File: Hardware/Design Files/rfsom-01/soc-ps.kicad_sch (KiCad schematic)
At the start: 50 parts, among them J9 DM3CS-SF, U5 XC7Z010-1CLG400C, U7 TXS02612RTWR

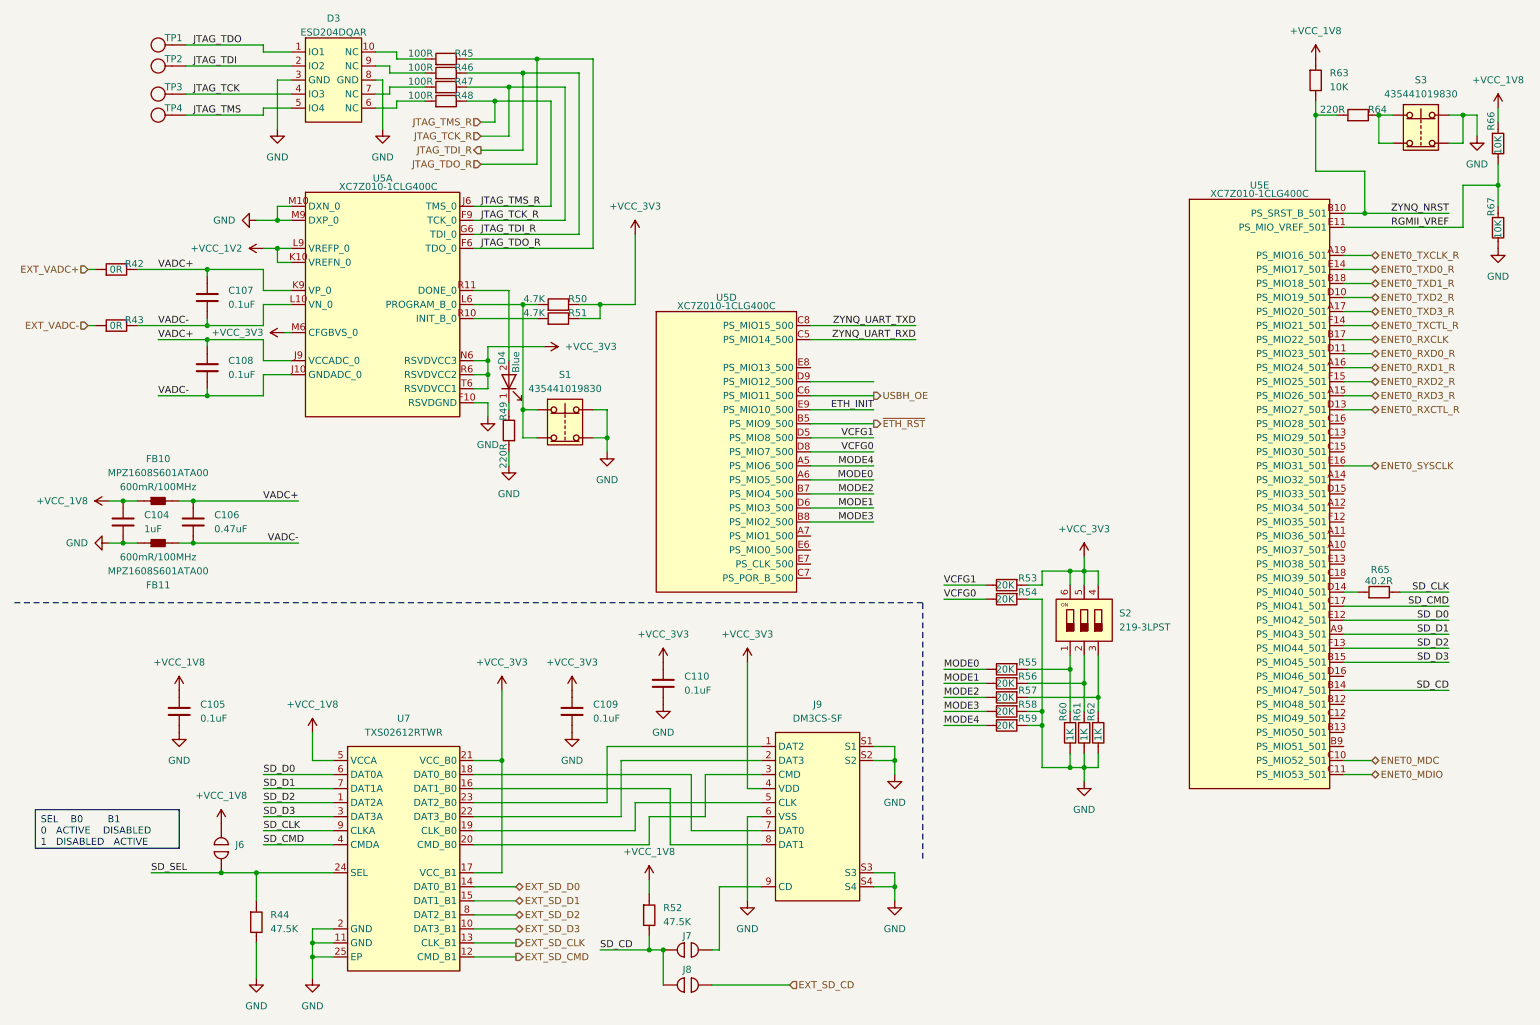
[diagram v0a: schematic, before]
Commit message: added starage, usb sch; more design progress in sch;
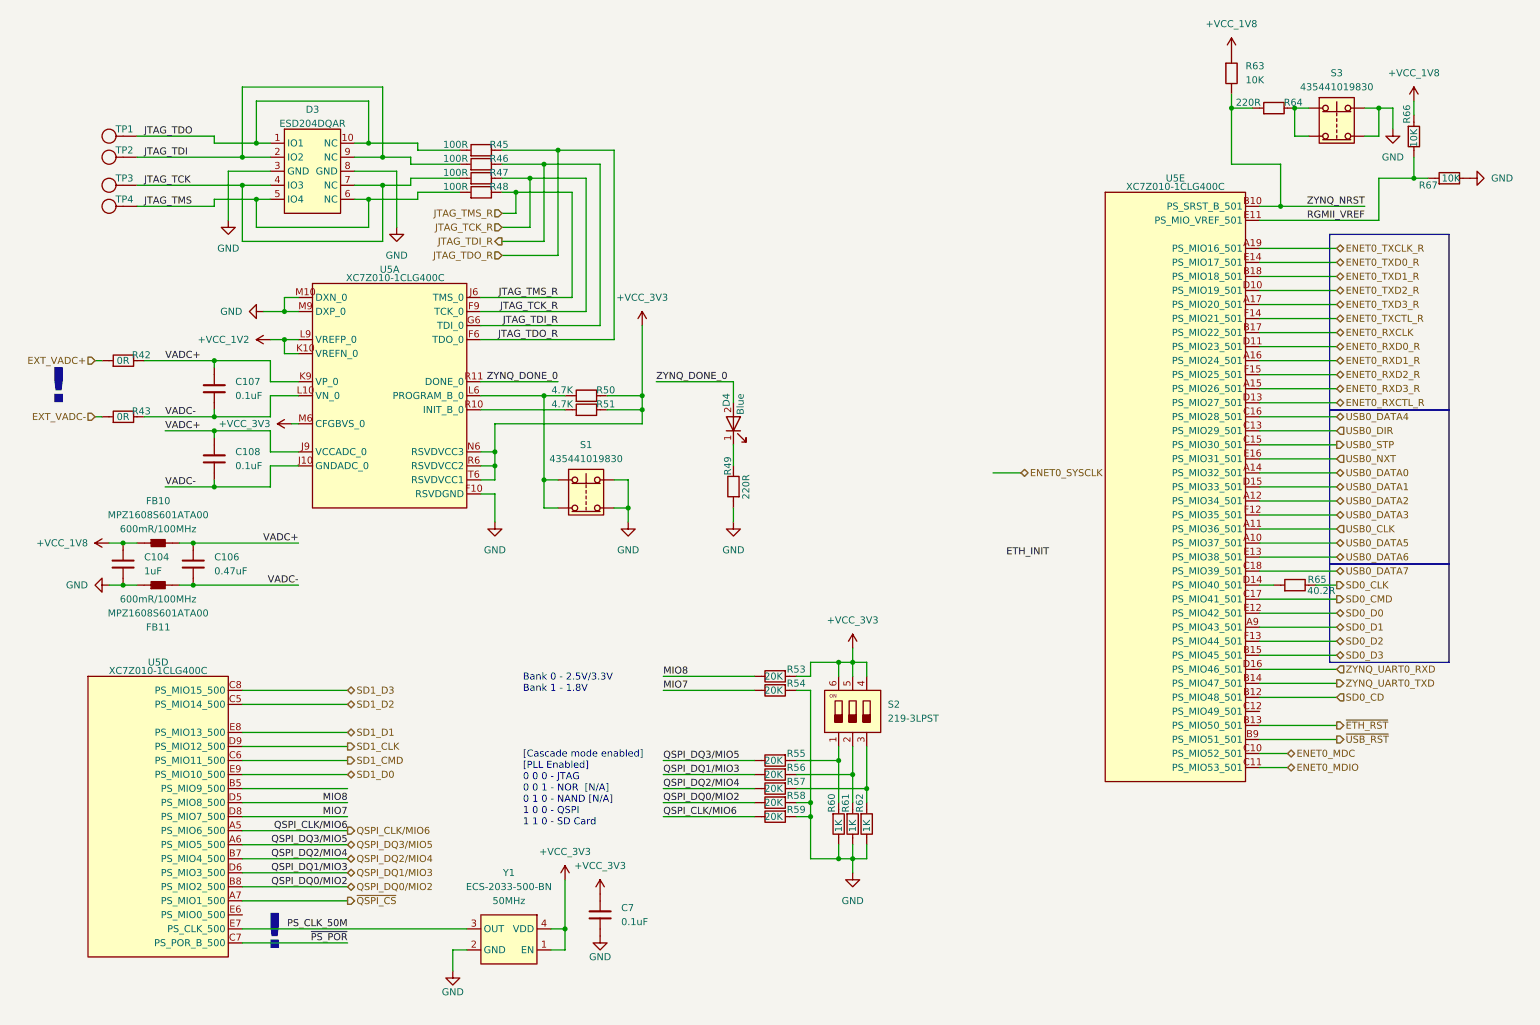
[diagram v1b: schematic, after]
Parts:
- removed C105, C109, C110: CL05B104KA5NNNC, Capacitor_SMD:C_0402_1005Metric, symbol Capacitors:CL05B104KA5NNNC
- removed J6, J7, J8: ~, Jumper:SolderJumper-2_P1.3mm_Open_RoundedPad1.0x1.5mm, symbol Miscellaneous:JMP_SLD
- removed J9: DM3CS-SF, Connectors:DM3CS-SF, symbol Connectors:DM3CS-SF
- removed R44, R52: RC0603FR-0747K5L, Resistor_SMD:R_0603_1608Metric, symbol Resistors:RC0603FR-0747K5L
- removed U7: TXS02612RTWR, ICs:QFN-24-1EP_4x4mm_P0.5mm, symbol ICs:TXS02612RTWR
- added C7: CL05B104KA5NNNC, Capacitor_SMD:C_0402_1005Metric, symbol Capacitors:CL05B104KA5NNNC
- added Y1: ECS-2033-500-BN, Miscellaneous:ECS-2033, symbol Miscellaneous:ECS-2033-500-BN
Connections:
- net +VCC_3V3: now also C7.1, Y1.1 (EN), Y1.4 (VDD)
- net ENET0_SYSCLK: no longer U5.E16 (PS_MIO31_501)
- net ETH_INIT: no longer U5.E9 (PS_MIO10_500)
- net GND: now also C7.2, Y1.2 (GND)
- net JTAG_TCK: now also D3.7 (NC), R47.1
- net JTAG_TDI: now also D3.9 (NC), R46.1
- net JTAG_TDO: now also D3.10 (NC), R45.1
- net JTAG_TMS: now also D3.6 (NC), R48.1
- net ~{ETH_RST}: now also U5.B13 (PS_MIO50_501); no longer U5.B5 (PS_MIO9_500)
- net ZYNQ_DONE_0: now reaches D4.2 (A), U5.R11 (DONE_0)
- net USB0_DATA5: now reaches U5.A10 (PS_MIO37_501)
- net USB0_CLK: now reaches U5.A11 (PS_MIO36_501)
- net USB0_DATA2: now reaches U5.A12 (PS_MIO34_501)
- net USB0_DATA0: now reaches U5.A14 (PS_MIO32_501)
- net SD0_CD: now reaches U5.B12 (PS_MIO48_501)
- net ~{USB_RST}: now reaches U5.B9 (PS_MIO51_501)
- net USB0_DIR: now reaches U5.C13 (PS_MIO29_501)
- net USB0_STP: now reaches U5.C15 (PS_MIO30_501)
- net USB0_DATA4: now reaches U5.C16 (PS_MIO28_501)
- net USB0_DATA7: now reaches U5.C18 (PS_MIO39_501)
- net USB0_DATA1: now reaches U5.D15 (PS_MIO33_501)
- net ZYNQ_UART0_RXD: now reaches U5.D16 (PS_MIO46_501)
- net USB0_DATA6: now reaches U5.E13 (PS_MIO38_501)
- net USB0_DATA3: now reaches U5.F12 (PS_MIO35_501)
- net ~{QSPI_CS}: now reaches U5.A7 (PS_MIO1_500)
- net ~{PS_POR}: now reaches U5.C7 (PS_POR_B_500)
- net SD1_CLK: now reaches U5.D9 (PS_MIO12_500)
- net PS_CLK_50M: now reaches U5.E7 (PS_CLK_500)
- net PS_CLK_50M: now also Y1.3 (OUT)
- net SD1_D1: now reaches U5.E8 (PS_MIO13_500)
- net MODE0 renamed QSPI_DQ3/MIO5
- net MODE1 renamed QSPI_DQ1/MIO3
- net MODE2 renamed QSPI_DQ2/MIO4
- net MODE3 renamed QSPI_DQ0/MIO2
- net MODE4 renamed QSPI_CLK/MIO6
- net SD_CD renamed ZYNQ_UART0_TXD
- net SD_CLK renamed SD0_CLK
- net SD_CMD renamed SD0_CMD
- net SD_D0 renamed SD0_D0
- net SD_D1 renamed SD0_D1
- net SD_D2 renamed SD0_D2
- net SD_D3 renamed SD0_D3
- net USBH_OE renamed SD1_CMD
- net VCFG0 renamed MIO7
- net VCFG1 renamed MIO8
- net ZYNQ_UART_RXD renamed SD1_D2
- net ZYNQ_UART_TXD renamed SD1_D3
- new net SD1_D0: U5.E9 (PS_MIO10_500)
- new net USB0_NXT: U5.E16 (PS_MIO31_501)
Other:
- note added: "!"
- note added: "Bank 0 - 2.5V/3.3V Bank 1 - 1.8V"
- note added: "[Cascade mode enabled] [PLL Enabled] 0 0 0 - JTAG 0 0 1 - NOR [N/A] 0 1 0 - NAND [N/A] 1 0 0 - QSPI 1 1 0 - SD Card"
- moved on the sheet: C104, C106, C107, C108, D3, D4, FB10, FB11, R42, R43, R45, R46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
